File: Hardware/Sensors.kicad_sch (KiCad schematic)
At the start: 3 parts, among them U4 BMP581, U5 BMM350, U6 BMI088

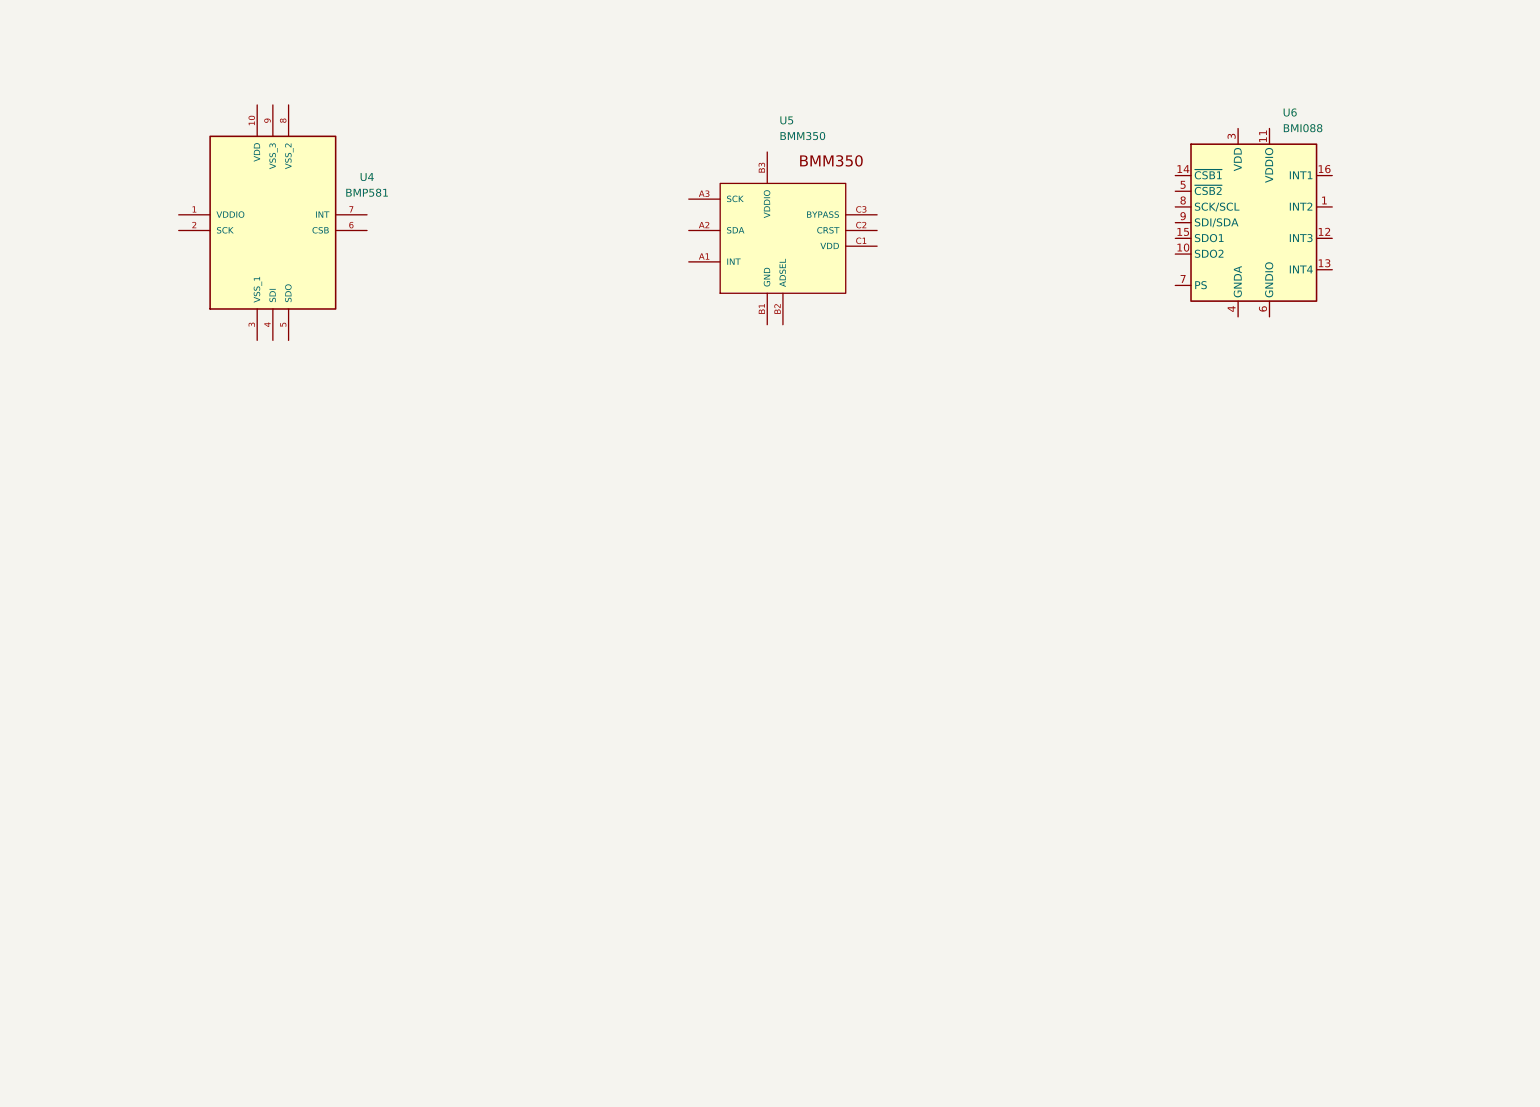
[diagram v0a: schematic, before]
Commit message: 19-feb update
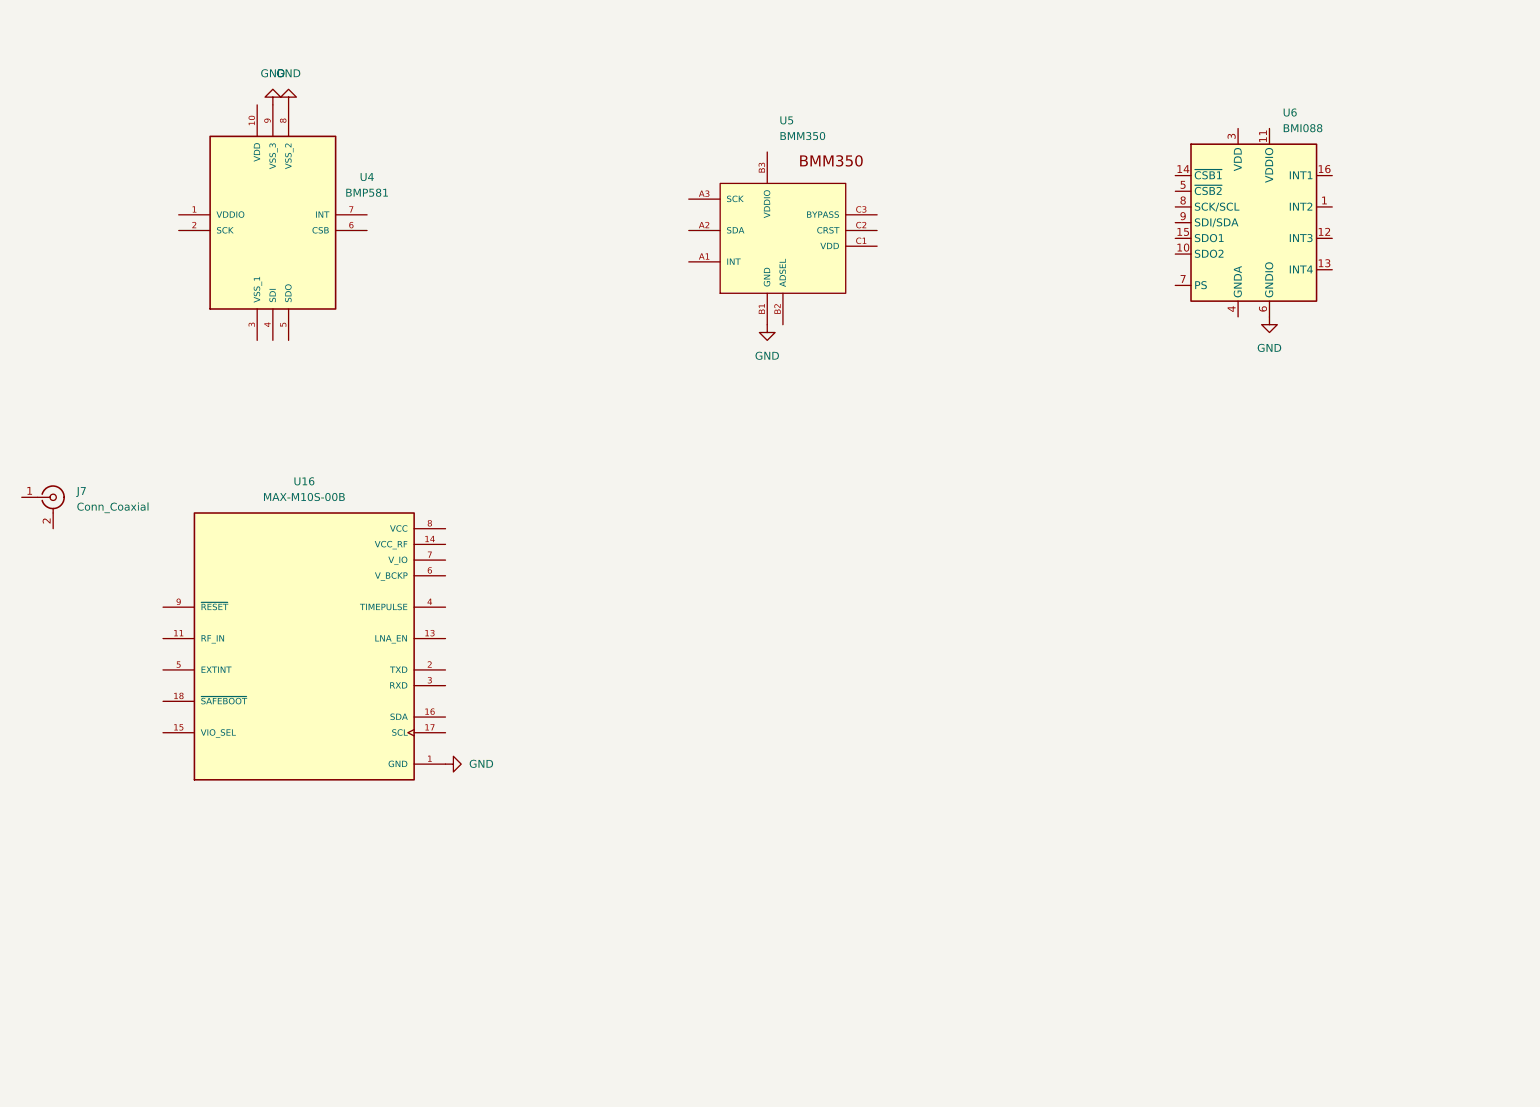
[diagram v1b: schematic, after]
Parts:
- added J7: Conn_Coaxial, Connector_Coaxial:SMA_Amphenol_901-143_Horizontal, symbol Connector:Conn_Coaxial
- added U16: MAX-M10S-00B, MAX-M10S-00B:XCVR_MAX-M10S-00B, symbol MAX-M10S-00B:MAX-M10S-00B
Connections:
- net GND: now reaches U6.6 (GNDIO)
- net GND: now also U4.8 (VSS_2), U4.9 (VSS_3), U5.B1 (GND), U16.1 (GND), U16.10 (GND), U16.12 (GND)

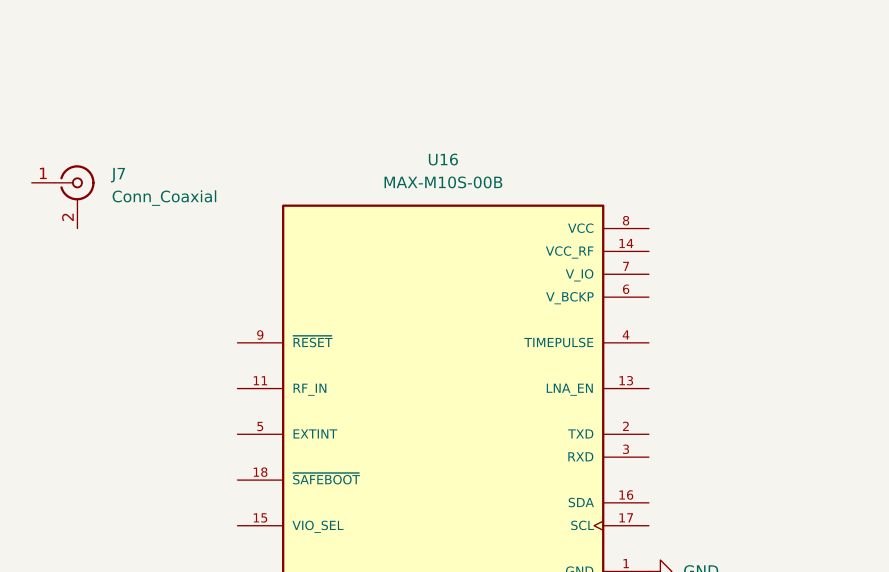
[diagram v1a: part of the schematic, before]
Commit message: 27 feb update
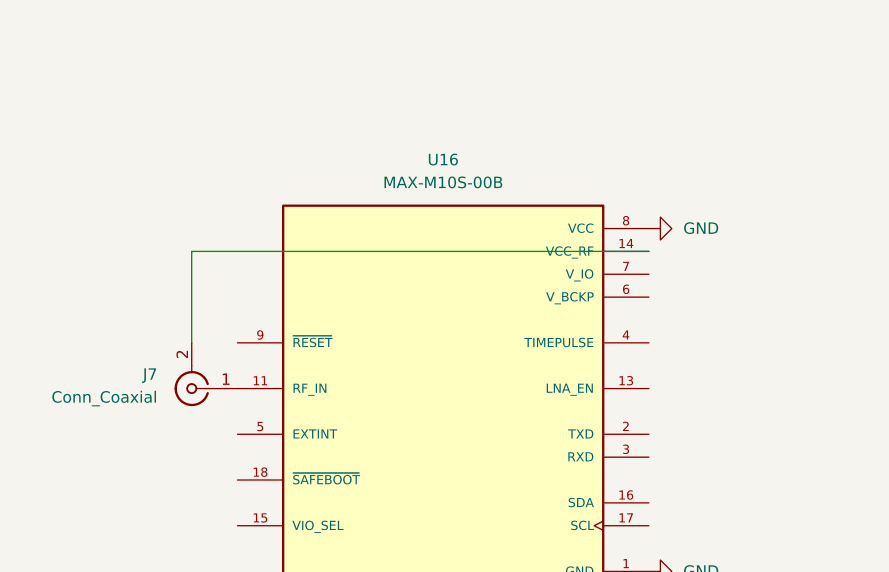
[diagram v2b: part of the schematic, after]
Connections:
- net GND: now also U16.8 (VCC)
- net at J7.1 (In): now also U16.11 (RF_IN)
- net at J7.2 (Ext): now also U16.14 (VCC_RF)
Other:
- moved on the sheet: J7
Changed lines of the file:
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@@
 	(title_block
 		(title "Blitz")
+		(date "2026-02-19")
+	)
+	(wire
+		(pts
+			(xy 40.64 100.33) (xy 91.44 100.33)
+		)
+		(stroke
+			(width 0)
+			(type default)
+		)
+	)
+	(wire
+		(pts
+			(xy 40.64 110.49) (xy 40.64 100.33)
+		)
+		(stroke
+			(width 0)
+			(type default)
+		)
 	)
 	(symbol
@@
 	(symbol
 		(lib_id "Connector:Conn_Coaxial")
-		(at 27.94 92.71 0)
+		(at 40.64 115.57 180)
 		(unit 1)
 		(exclude_from_sim no)
@@
 		(fields_autoplaced yes)
 		(property "Reference" "J7"
-			(at 31.75 91.7331 0)
+			(at 36.83 114.0067 0)
 			(effects
 				(font
@@
 		)
 		(property "Value" "Conn_Coaxial"
-			(at 31.75 94.2731 0)
+			(at 36.83 116.5467 0)
 			(effects
 				(font
@@
 		)
 		(property "Footprint" "Connector_Coaxial:SMA_Amphenol_901-143_Horizontal"
-			(at 27.94 92.71 0)
+			(at 40.64 115.57 0)
 			(effects
 				(font
@@
 		)
 		(property "Datasheet" "~"
-			(at 27.94 92.71 0)
+			(at 40.64 115.57 0)
 			(effects
 				(font
@@
 		)
 		(property "Description" "coaxial connector (BNC, SMA, SMB, SMC, Cinch/RCA, LEMO, ...)"
-			(at 27.94 92.71 0)
+			(at 40.64 115.57 0)
 			(effects
 				(font
@@
 					(unit 1)
 				)
+			)
+		)
+	)
+	(symbol
+		(lib_id "power:GND")
+		(at 91.44 97.79 90)
+		(unit 1)
+		(exclude_from_sim no)
+		(in_bom yes)
+		(on_board yes)
+		(dnp no)
+		(fields_autoplaced yes)
+		(property "Reference" "#PWR096"
+			(at 97.79 97.79 0)
+			(effects
+				(font
+					(size 1.27 1.27)
+				)
+				(hide yes)
+			)
+		)
+		(property "Value" "GND"
+			(at 95.25 97.7899 90)
+			(effects
+				(font
+					(size 1.27 1.27)
+				)
+				(justify right)
+			)
+		)
+		(property "Footprint" ""
+			(at 91.44 97.79 0)
+			(effects
+				(font
+					(size 1.27 1.27)
+				)
+				(hide yes)
+			)
+		)
+		(property "Datasheet" ""
+			(at 91.44 97.79 0)
+			(effects
+				(font
+					(size 1.27 1.27)
+				)
+				(hide yes)
+			)
+		)
+		(property "Description" "Power symbol creates a global label with name \"GND\" , ground"
+			(at 91.44 97.79 0)
+			(effects
+				(font
+					(size 1.27 1.27)
+				)
+				(hide yes)
+			)
+		)
+		(pin "1"
+		)
+		(instances
+			(project "Blitz"
+				(path "/e8b263af-d576-40b7-a774-1c6d96794e54/15fd4c35-84c4-4d4c-9c2f-0c9be770baef"
+					(reference "#PWR096")
+					(unit 1)
+				)
